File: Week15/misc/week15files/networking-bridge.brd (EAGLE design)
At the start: 44.8 x 24.8 mm, 8 parts, among them J1ISP AVRISPSMD, J3BUS PINHD-2X2-SMD

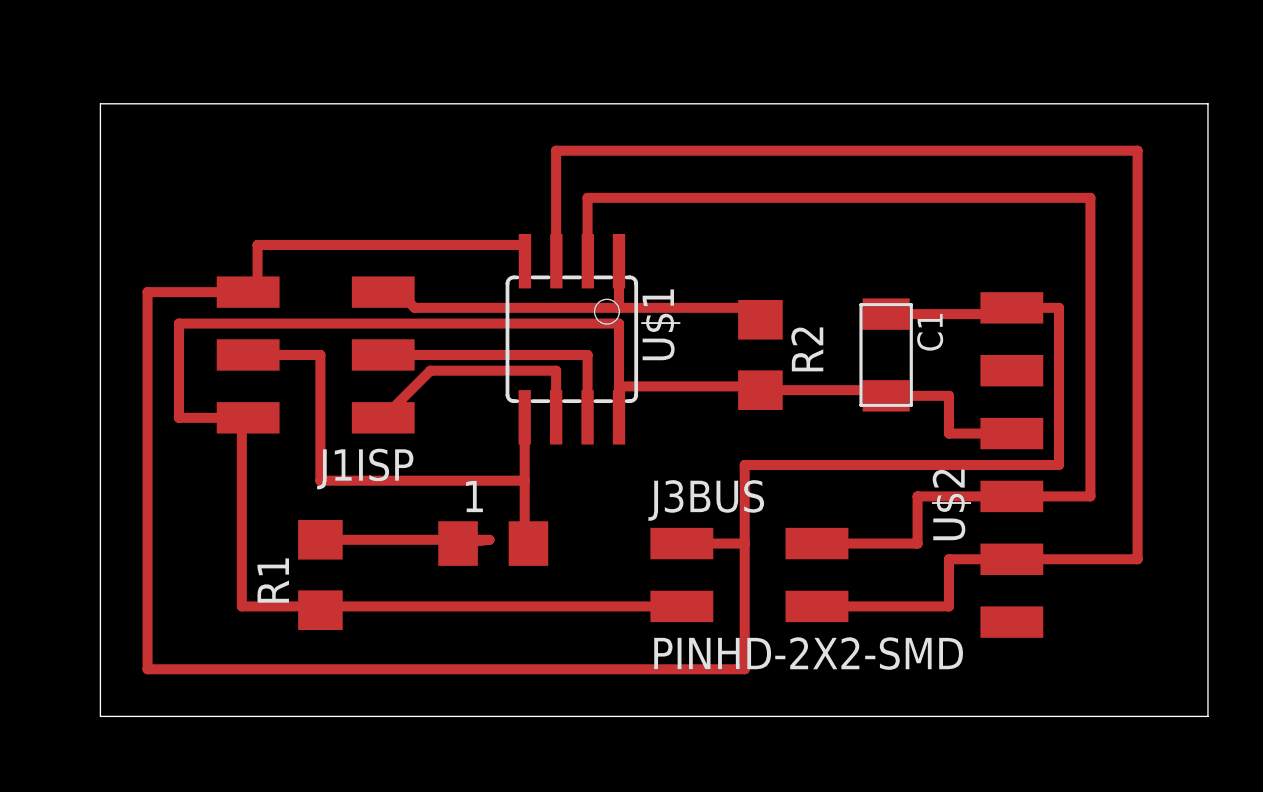
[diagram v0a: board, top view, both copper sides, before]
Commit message: week11/13/15/final
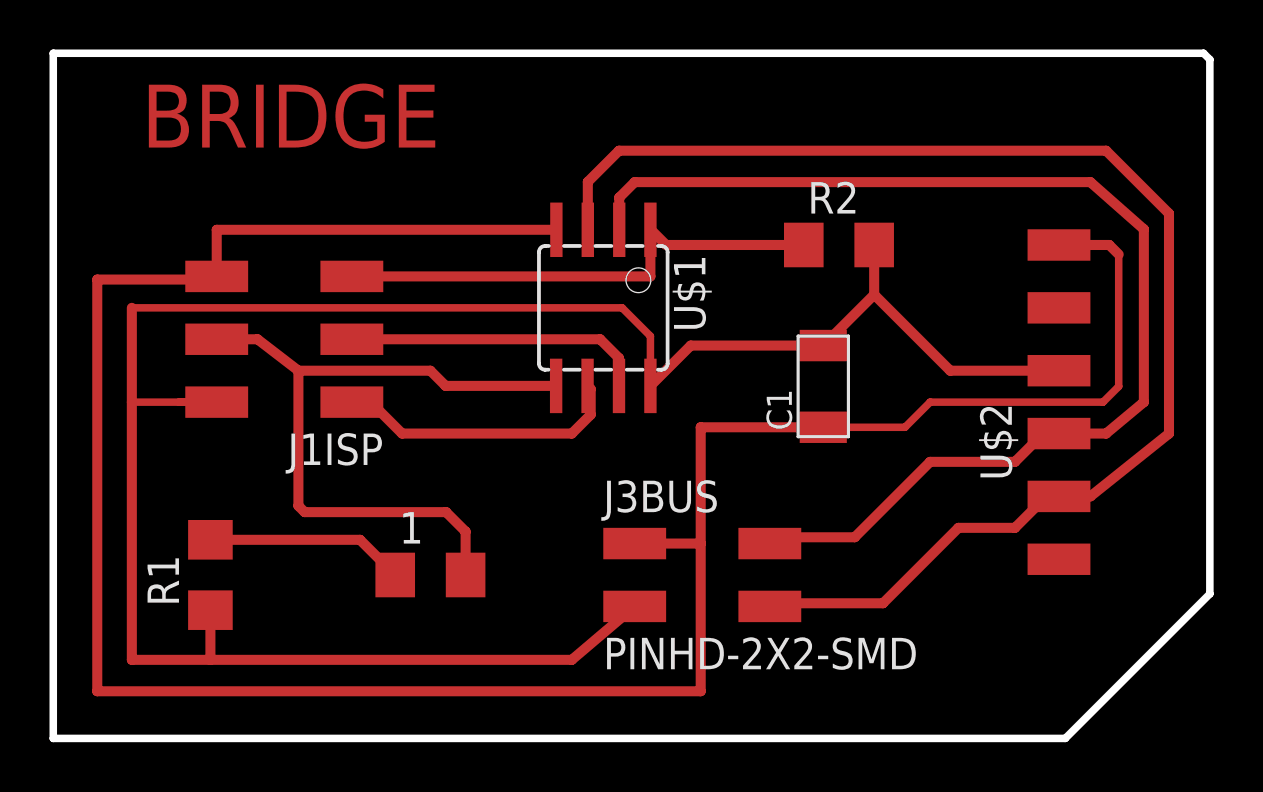
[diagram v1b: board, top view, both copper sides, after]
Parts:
- moved R2 5.46 mm to (29.8, 21.0), turned to 0 degrees
- moved R1 4.45 mm to (4.45, 7.62)
- moved U$2 3.18 mm to (38.7, 14.6)
- moved 1 2.84 mm to (13.3, 7.62)
- moved C1 2.84 mm to (29.2, 15.2), turned to 90 degrees
- moved J3BUS 1.91 mm to (24.1, 7.62)
- moved U$1 1.80 mm to (20.3, 18.4)
- moved J1ISP 1.42 mm to (7.62, 17.1)
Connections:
- removed net N$2: J1ISP.2, J3BUS.3
- removed net N$21: U$2.6
- net VCC: now also J1ISP.2, J3BUS.3, R1.1
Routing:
- net VCC: track 42.9 -> 87.1 mm
- net N$2: track 28.2 -> 0.00 mm
- net MOSI: track 22.1 -> 28.8 mm
- net GND: track 94.9 -> 100.7 mm
- net RX: track 59.3 -> 55.1 mm
- net RST: track 17.9 -> 20.4 mm
- net SCK: track 10.8 -> 13.0 mm
- net MISO: track 9.66 -> 11.7 mm
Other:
- board size 44.8 x 24.8 mm -> 46.7 x 27.7 mm
- board text added: "BRIDGE"
